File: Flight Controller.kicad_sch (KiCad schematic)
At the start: 123 parts, among them IC1 ICM-20689, IC2 AT7456E, J1 Micro_SD_Card, J2 USB_C_Receptacle_USB2.0_14P, Q1 BC817W, U1 STM32F405RGTx, U2 LMR51430, U3 BMP280, U4 NCP1117-3.3_SOT223

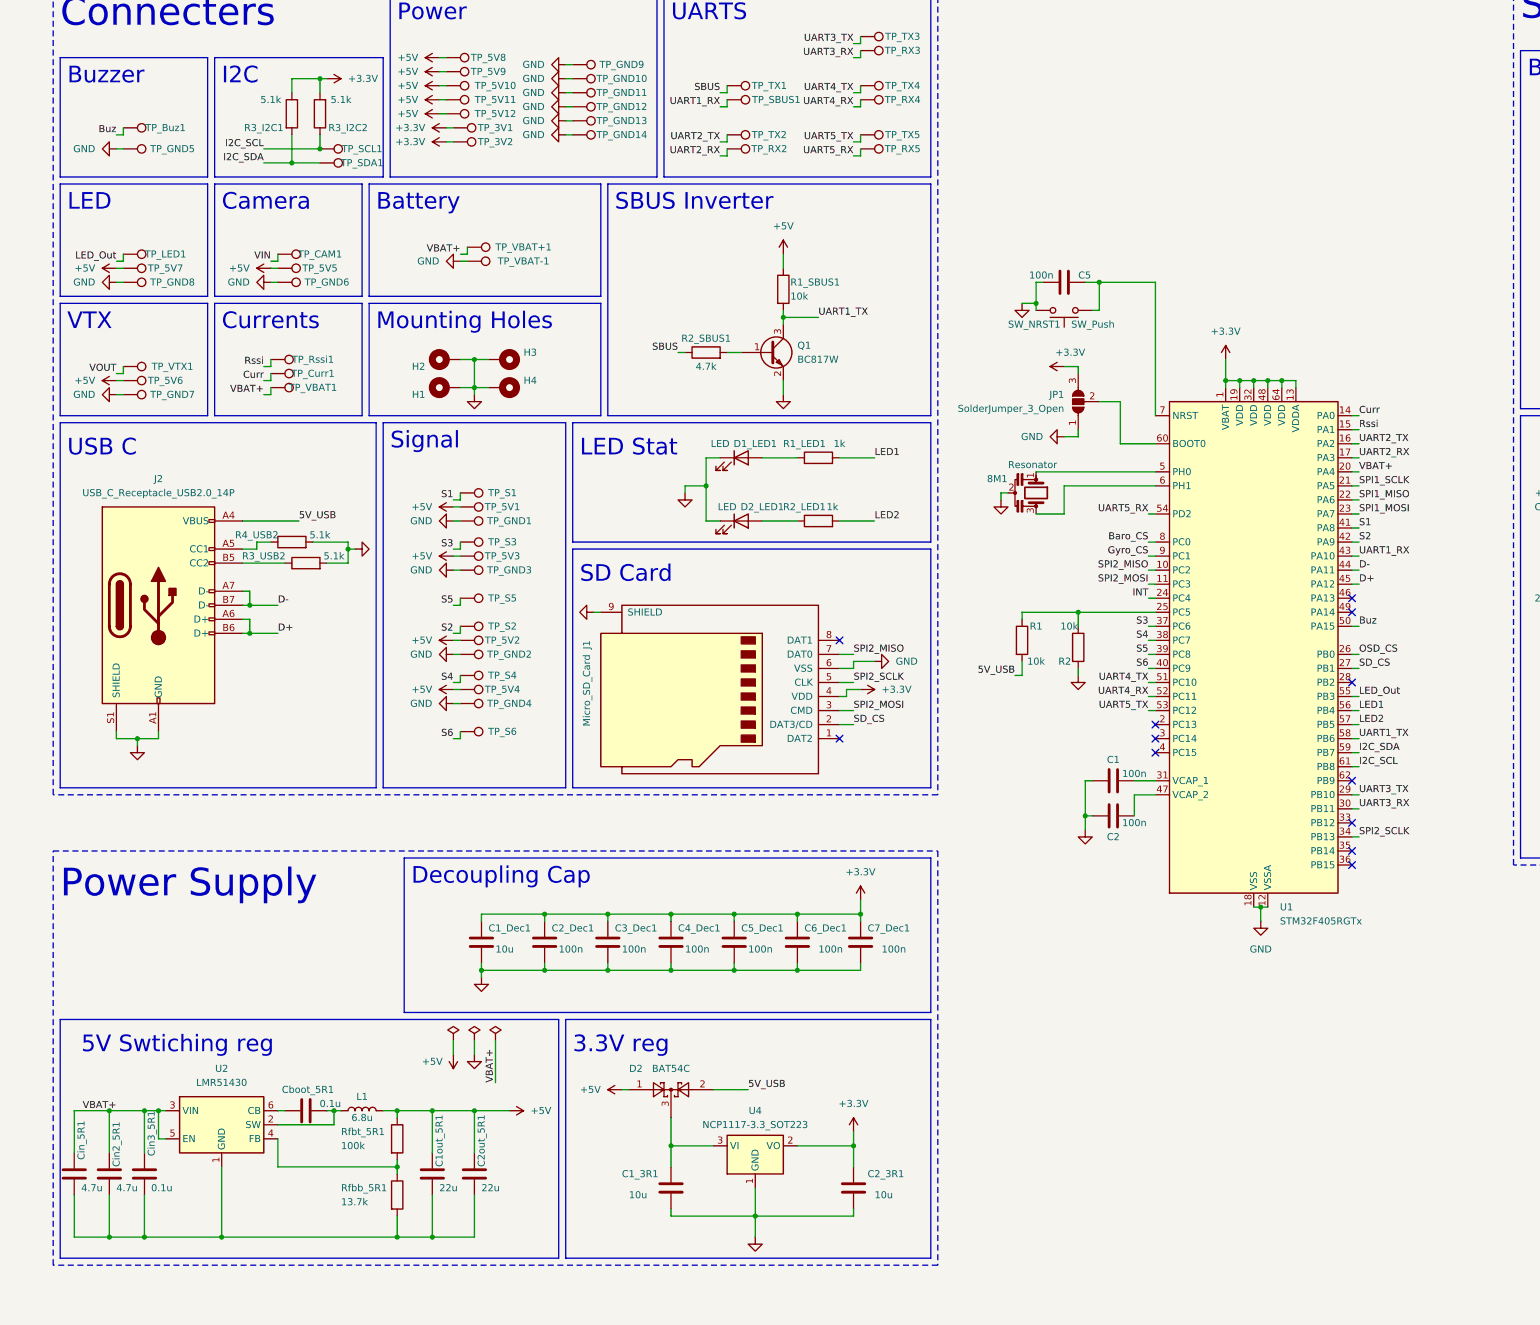
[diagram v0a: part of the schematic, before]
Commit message: Power Supply Sch Udpate
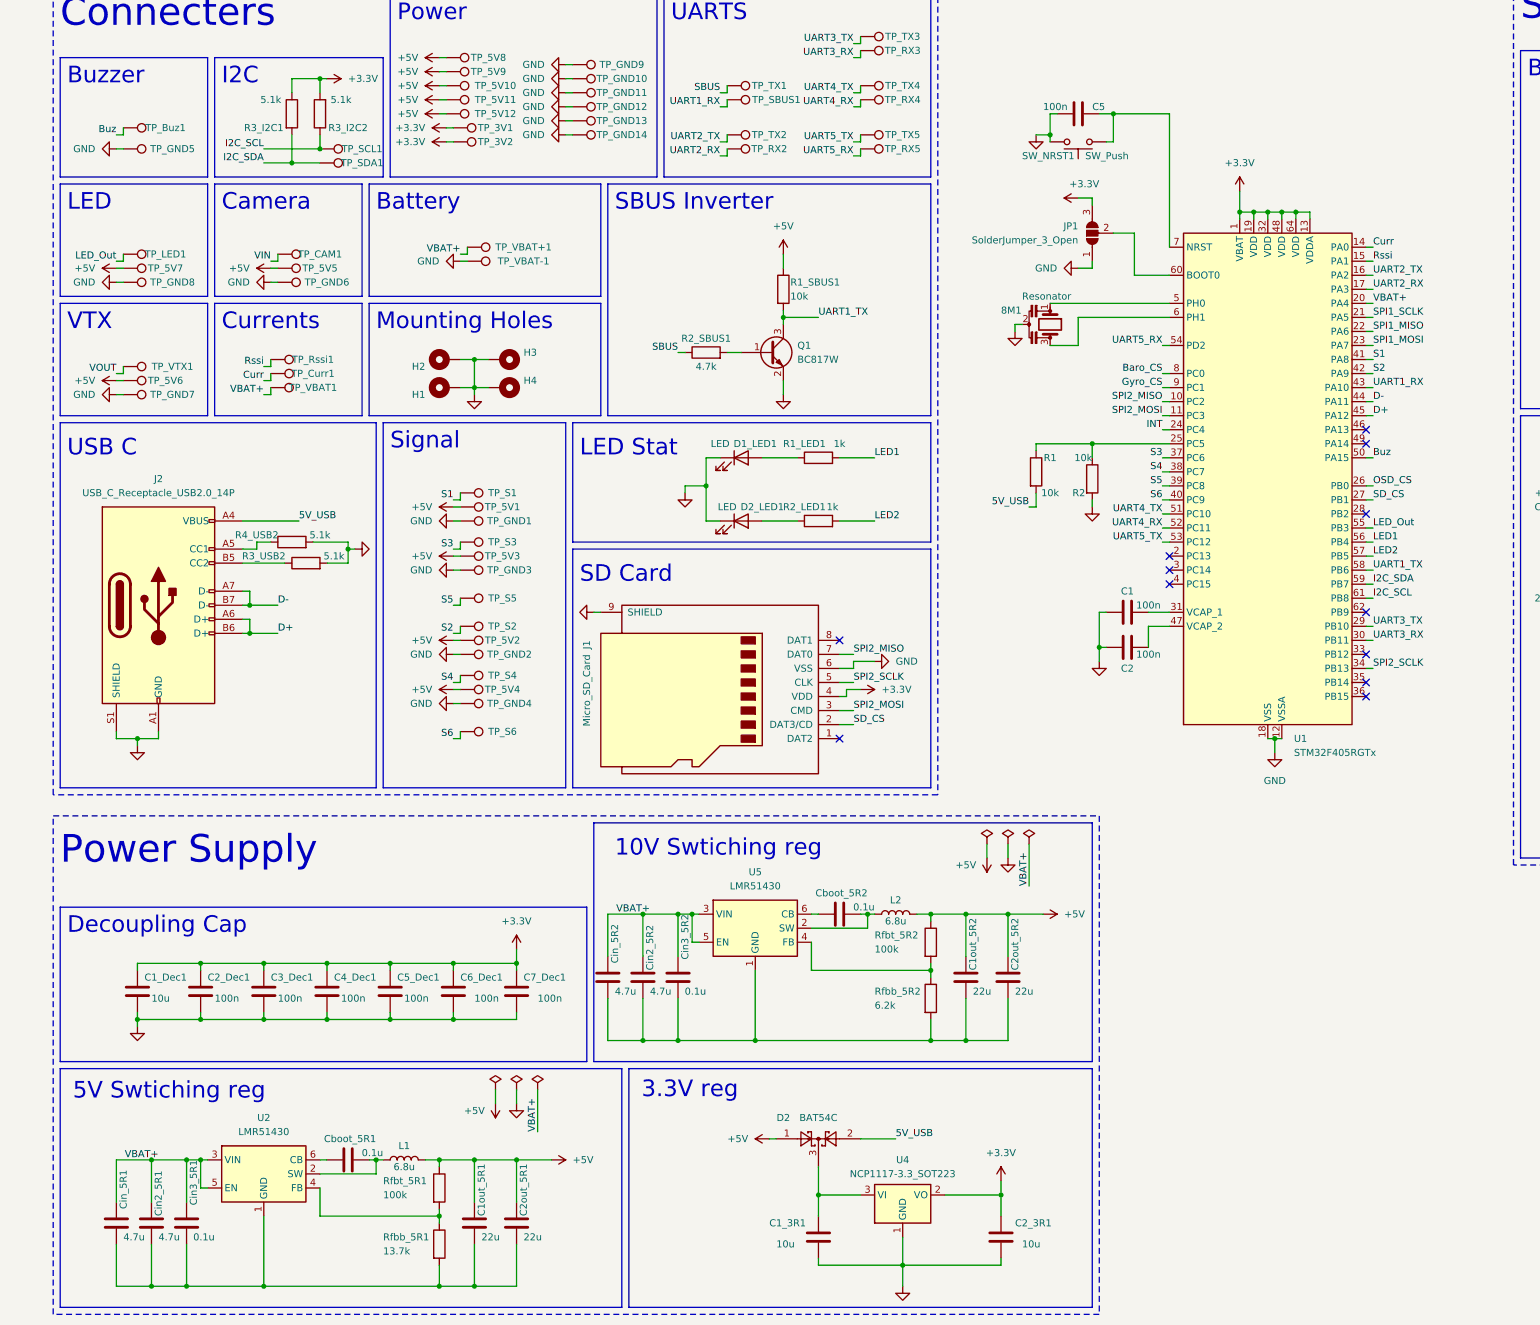
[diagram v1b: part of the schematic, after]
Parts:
- added C1out_5R2, C2out_5R2: 22u, Capacitor_SMD:C_0805_2012Metric, symbol Device:C
- added Cboot_5R2, Cin3_5R2: 0.1u, Capacitor_SMD:C_0402_1005Metric, symbol Device:C
- added Cin2_5R2, Cin_5R2: 4.7u, Capacitor_SMD:C_0805_2012Metric, symbol Device:C
- added L2: 6.8u, Inductor_SMD:L_Abracon_ASPI-0630LR, symbol Device:L
- added Rfbb_5R2: 6.2k, Resistor_SMD:R_0805_2012Metric, symbol Device:R
- added Rfbt_5R2: 100k, Resistor_SMD:R_1206_3216Metric, symbol Device:R
- added U5: LMR51430, Package_TO_SOT_SMD:SOT-23-6, symbol Regulator_Switching:LMR51430
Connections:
- net +5V: now also C1out_5R2.1, C2out_5R2.1, L2.2, Rfbt_5R2.1
- net VBAT+: now also Cin2_5R2.1, Cin3_5R2.2, Cin_5R2.1, U5.3 (VIN), U5.5 (EN)
- new net: C1out_5R2.2, C2out_5R2.2, Cin2_5R2.2, Cin3_5R2.1, Cin_5R2.2, Rfbb_5R2.2, U5.1 (GND)
- new net: Cboot_5R2.1, U5.6 (CB)
- new net: Cboot_5R2.2, L2.1, U5.2 (SW)
- new net: Rfbb_5R2.1, Rfbt_5R2.2, U5.4 (FB)
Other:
- note added: "10V Swtiching reg"
- moved on the sheet: 8M1, C1, C1_3R1, C1_Dec1, C1out_5R1, C2, C2_3R1, C2_Dec1, C2out_5R1, C3_Dec1, C4_Dec1, C5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
